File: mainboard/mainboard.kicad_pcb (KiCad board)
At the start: 2 copper layers, 44.3 x 46.2 mm, 107 parts, among them J1 USB_B_Micro, J2 Conn_01x02_MountingPin, J3 Conn_01x19_MountingPin, J4 Conn_01x19_MountingPin, Q1 DMG2301L, Q2 MMBT3904, Q3 MMBT3904, SW1 SW_Push, SW2 SW_Push, U1 tps63070, U2 tps63070, U3 tps63070, U4 BME680, U5 LIS3MDL, U6 BH1750FVI, U7 CP2102N-A01-GQFN24, U8 ESP32-WROOM-32, U9 ADXL343

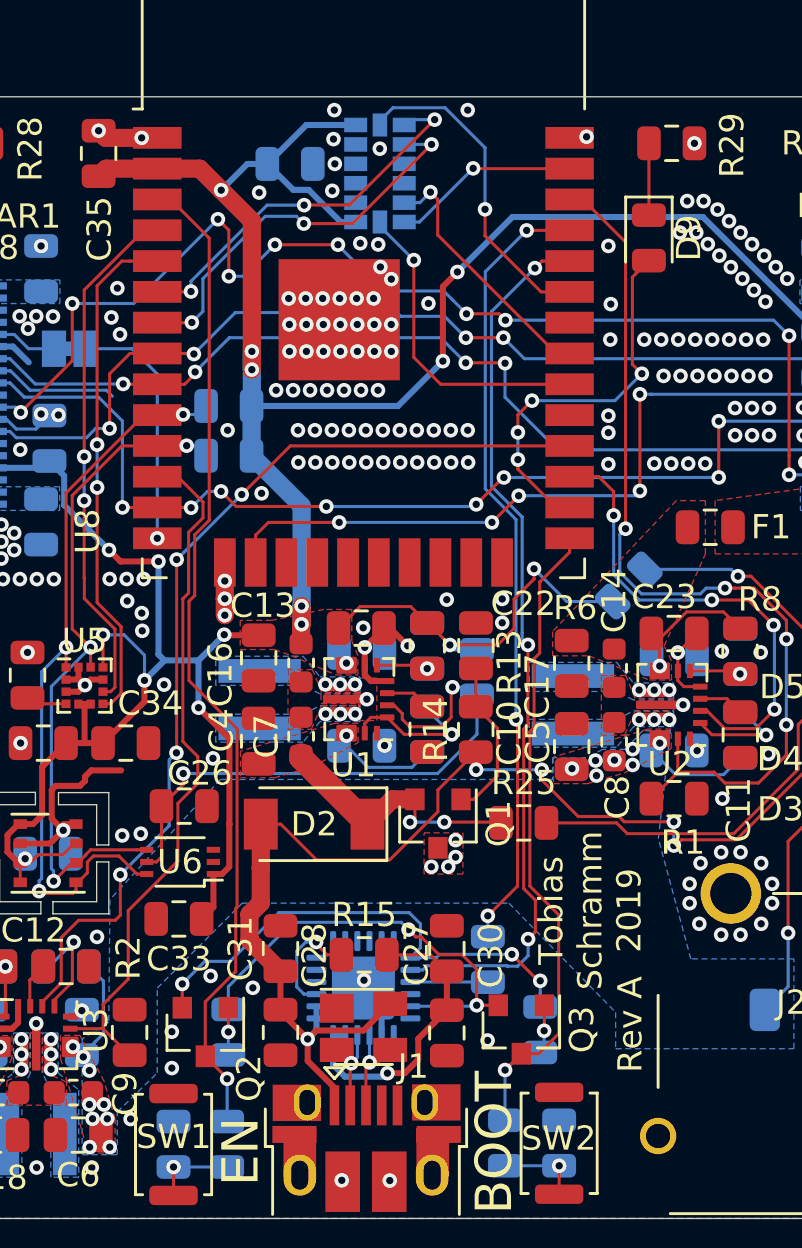
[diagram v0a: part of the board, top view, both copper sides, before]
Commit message: Replace reset circuitry
It was the reference circuit used on the DevKitC V4 but it just plain does not work.
Replaced by much simpler and more reliable design.
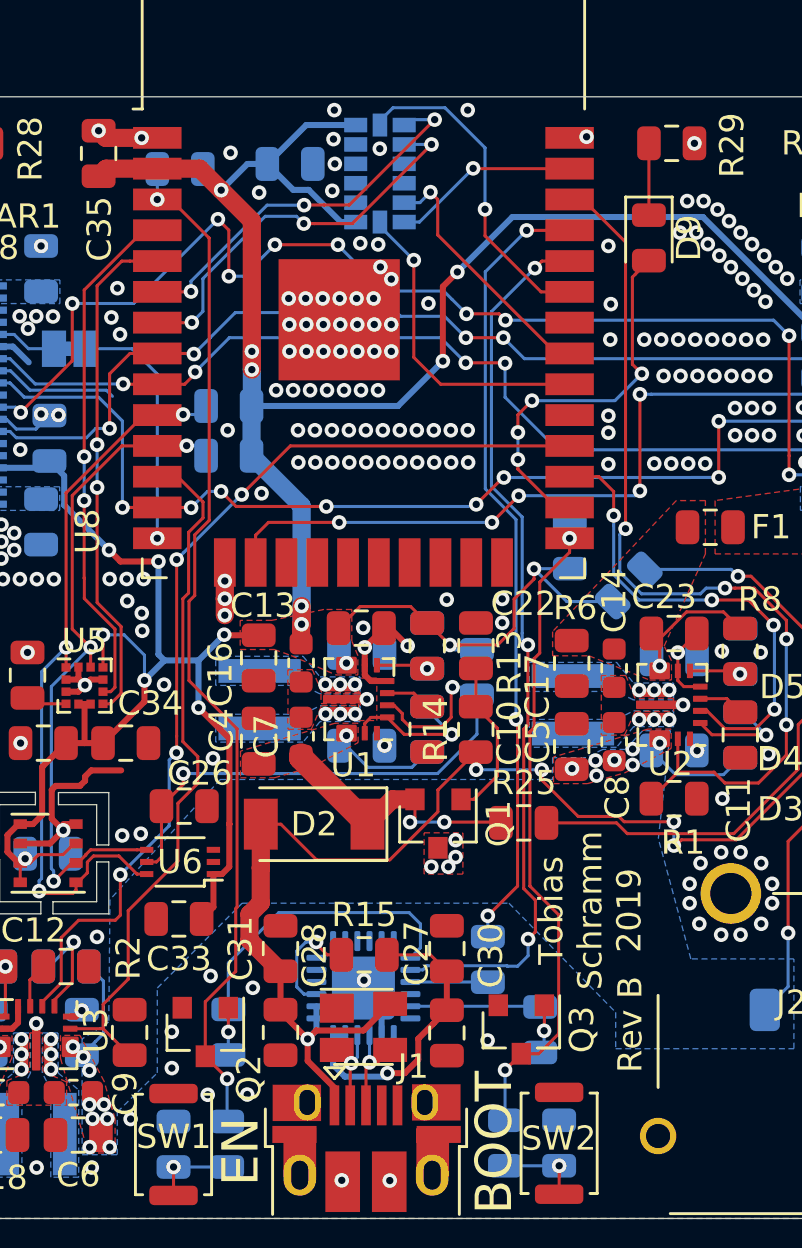
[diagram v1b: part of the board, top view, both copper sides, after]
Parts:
- added R30: 10 kR, Resistor_SMD:R_0805_2012Metric, B.Cu at (72.4, 86.7)
- added R31: 10 kR, Resistor_SMD:R_0805_2012Metric, B.Cu at (88.5, 102.3)
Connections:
- Q2 pad 2: /RTS -> GND
- Q3 pad 2: /DTR -> GND
- R17 pad 2: /DTR -> /RTS
- R18 pad 2: /RTS -> /DTR
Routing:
- net /DTR: track 18.2 -> 5.37 mm, vias 2 -> 0
- net /RTS: track 20.8 -> 12.5 mm, vias 3 -> 0
- net +3V3: track 139.6 -> 142.2 mm
- net /EN: track 41.3 -> 42.6 mm, vias 1 -> 2
- net /IO0: track 26.5 -> 27.1 mm, vias 1 -> 2
- net GND: track 55.0 -> 55.1 mm, vias 215 -> 218
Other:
- board text added: "Rev B"
- board text removed: "Rev A"

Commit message: Revert "Replace reset circuitry"
This reverts commit 4aa51ba1305b71722c80cb68cdfb79191ae487c4.

CP2102N defaults to RTS + CTS high. Thus the reference reset circuitry is the only
simple way to make this work
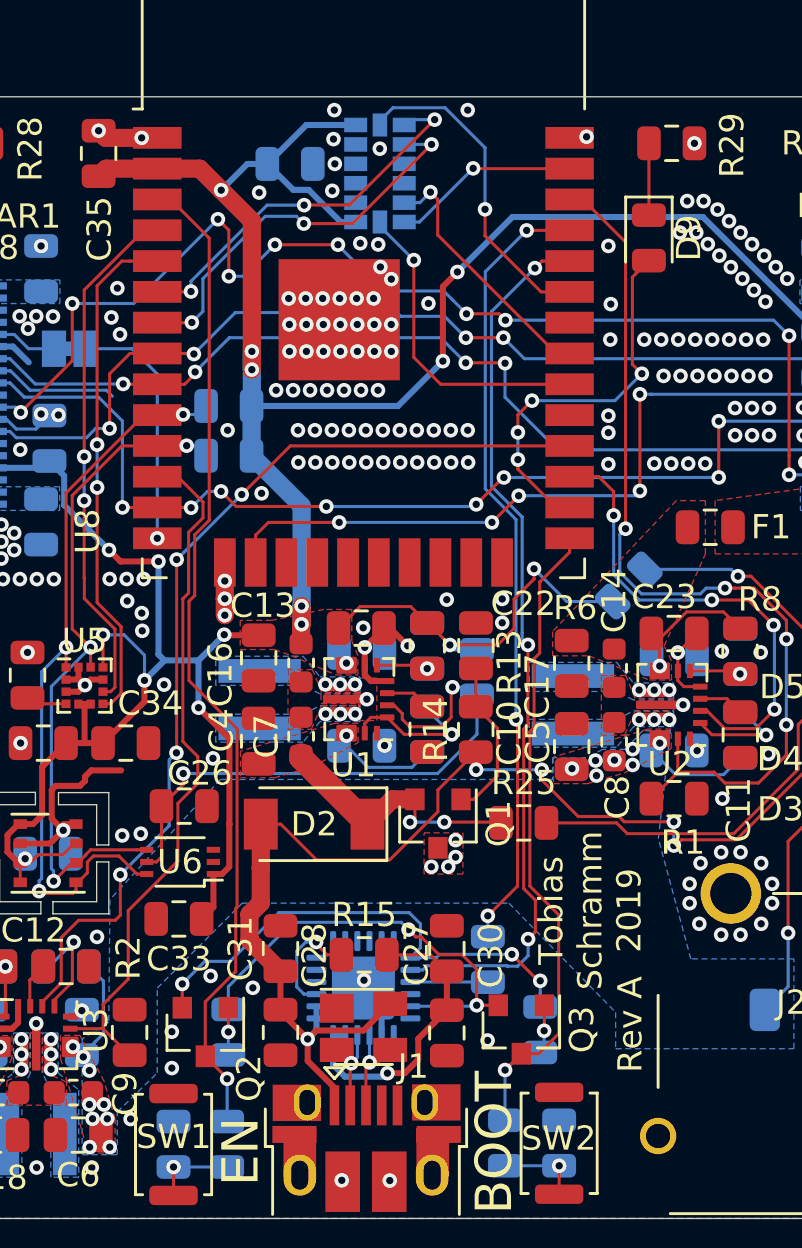
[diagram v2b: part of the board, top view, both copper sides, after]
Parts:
- removed R30, R31: 10 kR, Resistor_SMD:R_0805_2012Metric
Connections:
- Q2 pad 2: GND -> /RTS
- Q3 pad 2: GND -> /DTR
- R17 pad 2: /RTS -> /DTR
- R18 pad 2: /DTR -> /RTS
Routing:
- net /DTR: track 5.37 -> 18.2 mm, vias 0 -> 2
- net /RTS: track 12.5 -> 20.8 mm, vias 0 -> 3
- net +3V3: track 142.2 -> 139.6 mm
- net /EN: track 42.6 -> 41.3 mm, vias 2 -> 1
- net /IO0: track 27.1 -> 26.5 mm, vias 2 -> 1
- net GND: track 55.1 -> 55.0 mm, vias 218 -> 215
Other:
- board text added: "Rev A"
- board text removed: "Rev B"
